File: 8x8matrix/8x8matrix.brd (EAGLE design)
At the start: 60.4 x 60.5 mm, 18 parts

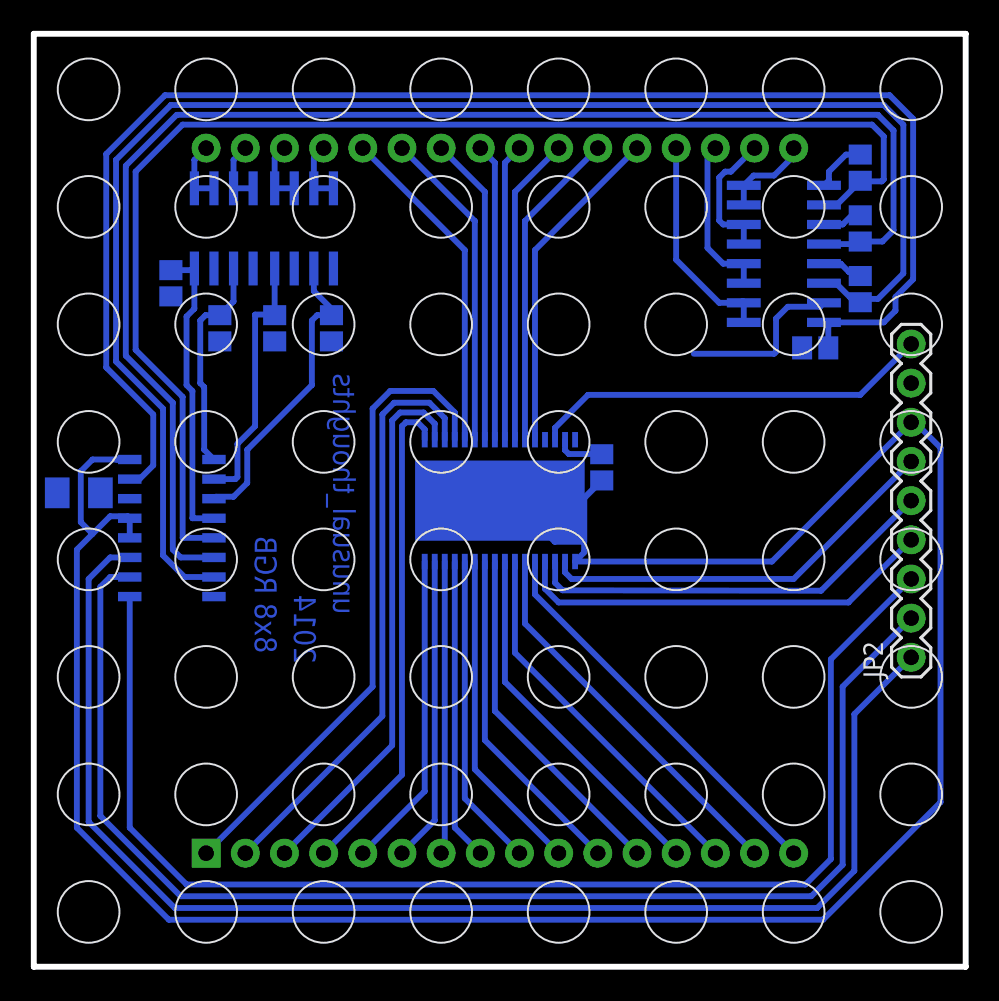
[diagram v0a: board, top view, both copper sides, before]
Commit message: reprint
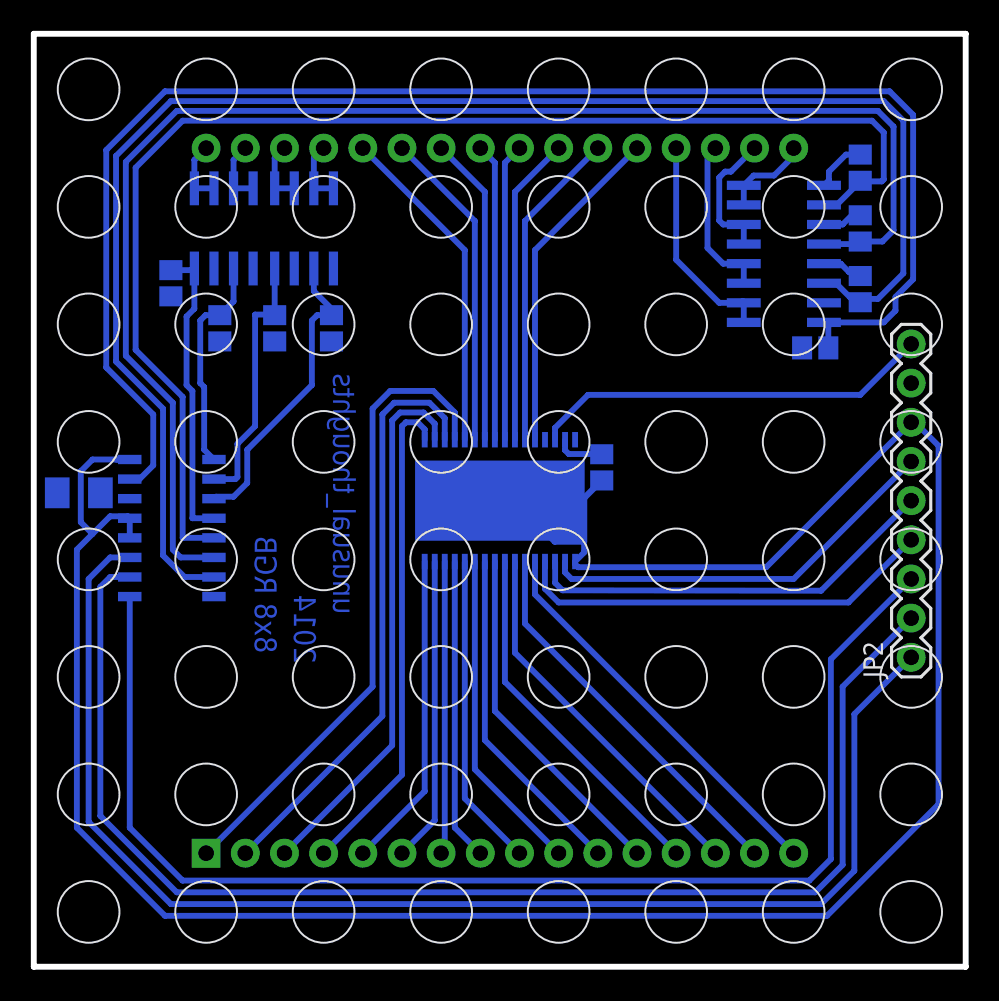
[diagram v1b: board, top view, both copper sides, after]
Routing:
- net 5.0V: track 19.8 -> 8.73 mm
- net Y1: track 92.0 -> 92.5 mm
- net Y7: track 97.5 -> 98.0 mm
- net Y2: track 84.5 -> 85.0 mm
- net Y0: track 100.0 -> 100.5 mm
